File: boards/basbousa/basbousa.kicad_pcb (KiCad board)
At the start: 2 copper layers, 133.4 x 90.7 mm, 25 parts

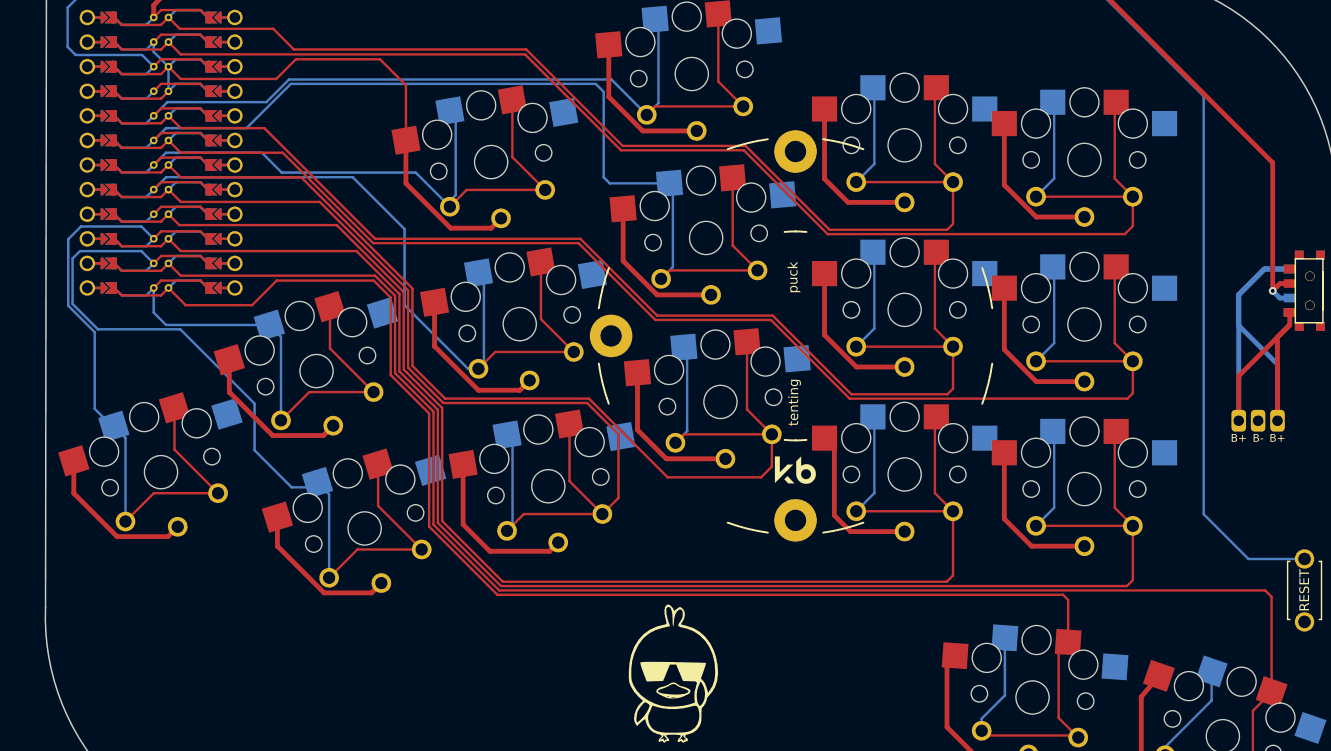
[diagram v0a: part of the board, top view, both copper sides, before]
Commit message: tighter basbousa
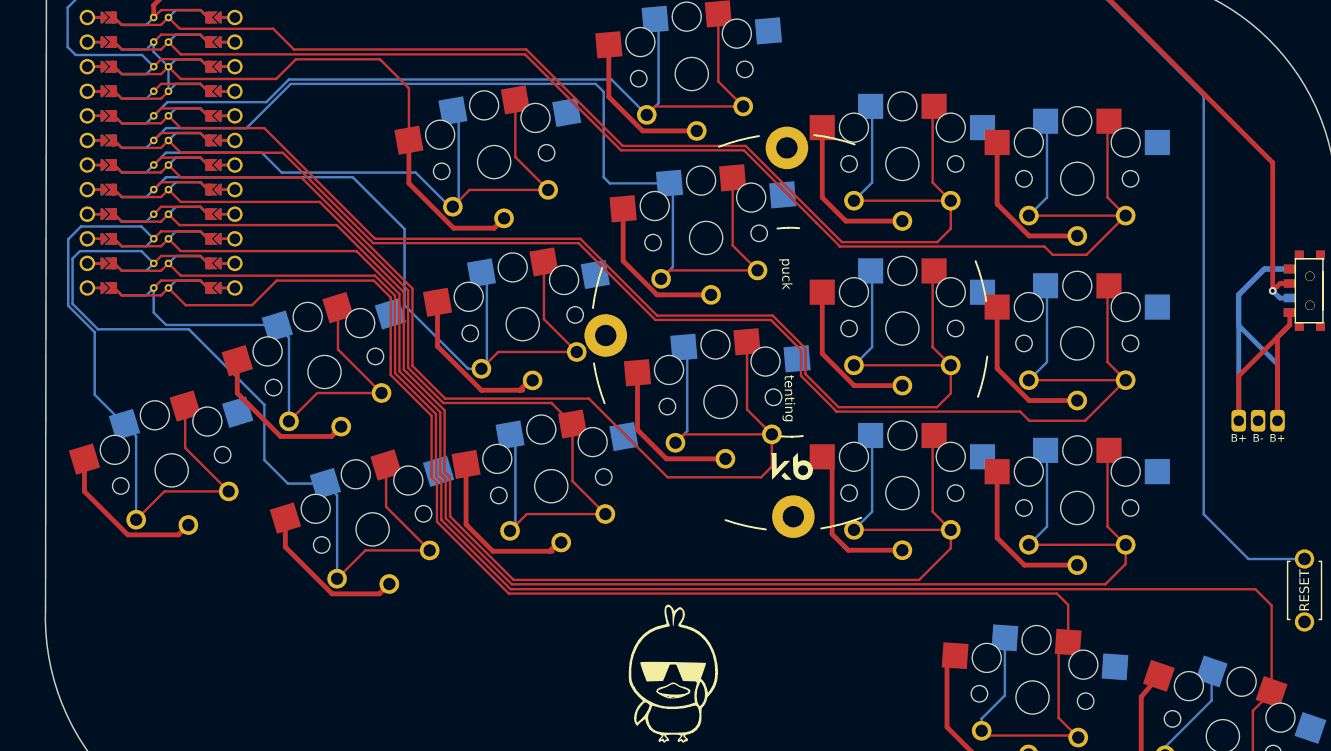
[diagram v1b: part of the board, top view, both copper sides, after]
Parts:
- moved S25 2.09 mm to (133.2, -69.2)
- moved S27 2.09 mm to (133.2, -86.2)
- moved S29 2.09 mm to (133.2, -103.2)
- moved S19 1.94 mm to (115.2, -70.8)
- moved S21 1.94 mm to (115.2, -87.8)
- moved S23 1.94 mm to (115.2, -104.8)
- moved S1 1.12 mm to (39.7, -73.1)
- moved S5 0.83 mm to (55.5, -83.3)
- moved S3 0.83 mm to (60.5, -67.0)
- moved REF** 0.67 mm to (103.6, -87.4), turned to 1 degrees
- moved S11 0.31 mm to (73.0, -105.0)
- moved S7 0.31 mm to (78.9, -71.5)
- moved S9 0.31 mm to (76.0, -88.2)
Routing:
- net P5: track 101.4 -> 87.3 mm
- net P6: track 146.7 -> 142.0 mm
- net P7: track 163.0 -> 158.4 mm
- net P16: track 81.1 -> 82.9 mm
- net P0: track 142.4 -> 141.0 mm
- net P8: track 181.8 -> 180.5 mm
- net P10: track 46.5 -> 47.7 mm
- net P9: track 156.2 -> 155.2 mm
- net P14: track 62.4 -> 63.2 mm
- net P1: track 126.2 -> 125.4 mm
- net P2: track 129.0 -> 129.8 mm
- net P18: track 78.5 -> 77.7 mm
